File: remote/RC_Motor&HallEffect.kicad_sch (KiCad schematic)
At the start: 9 parts, among them P2 JST CONN, Q1 NMOS, SW4 Button, U4 TMAG5253

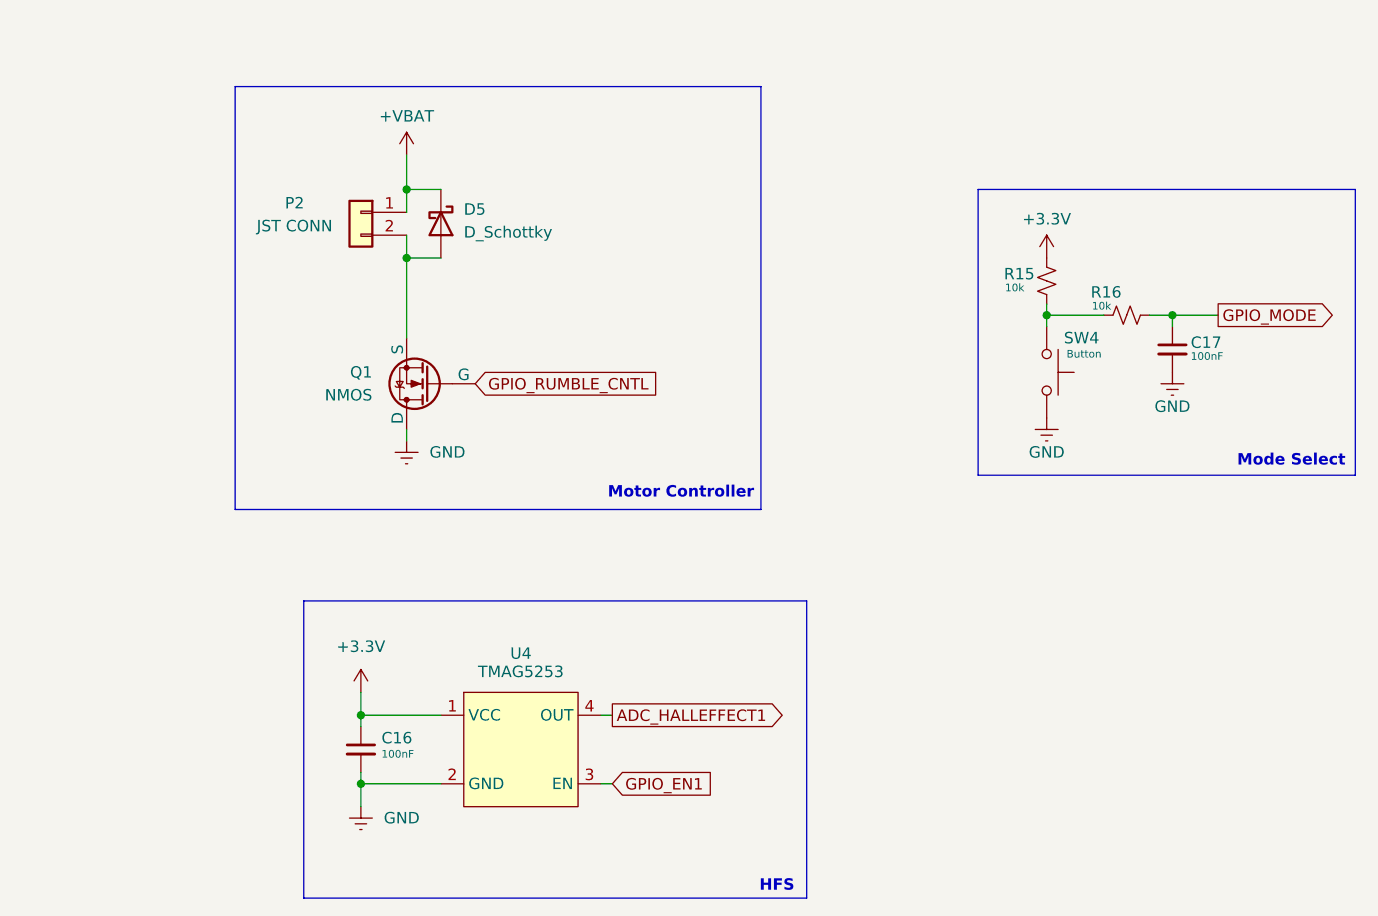
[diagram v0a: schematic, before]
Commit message: CRC V3
V 3.0.0
Initial version of CRC V3, fully redesigned remote
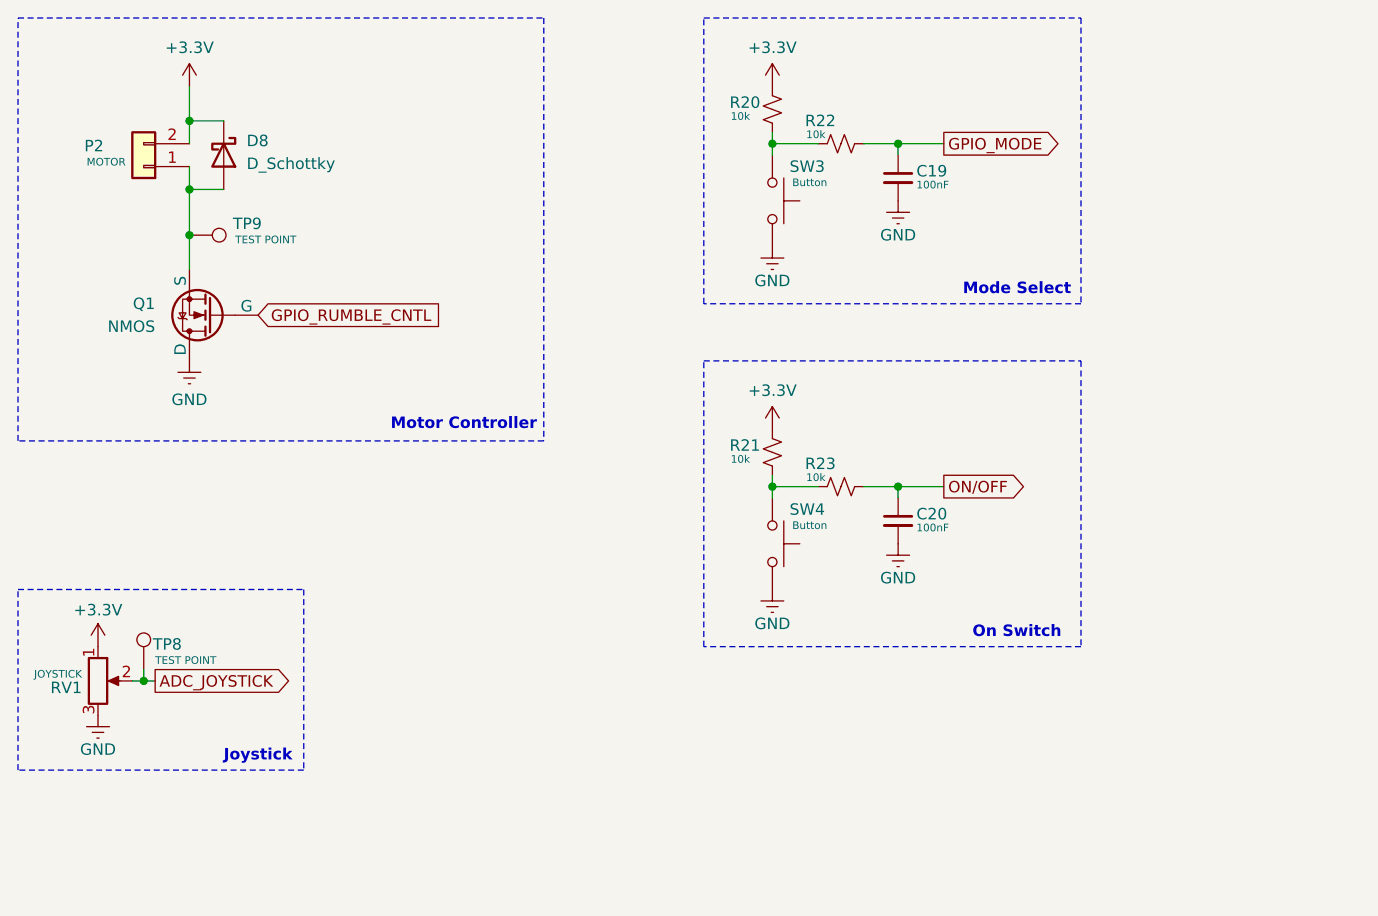
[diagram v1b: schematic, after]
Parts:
- removed C16: 100nF, Capacitor_SMD:C_0402_1005Metric, symbol Device:C_Small
- removed U4: TMAG5253, footprints:X2SON4_DMR_TEX, symbol New_Library_0:TMAG5253_Linear_Hall_Effect_Sensor
- added C20: 100nF, Capacitor_SMD:C_0402_1005Metric_Pad0.74x0.62mm_HandSolder, symbol Device:C_Small
- added R21, R23: 10k, Resistor_SMD:R_0402_1005Metric_Pad0.72x0.64mm_HandSolder, symbol Device:R_Small_US
- added RV1: JOYSTICK, footprints:Joystick Potentiometer Pads, symbol Device:R_Potentiometer
- added SW4: Button, footprints:Box Tactile Button Switch, symbol Switch:SW_Push
- added TP8, TP9: TEST POINT, TestPoint:TestPoint_Pad_2.0x2.0mm, symbol Connector:TestPoint
- C19: renamed from C17; footprint Capacitor_SMD:C_0402_1005Metric -> Capacitor_SMD:C_0402_1005Metric_Pad0.74x0.62mm_HandSolder
- P2: value JST CONN -> MOTOR; footprint footprints:CONN-SMD_2P-P2.00_XUNPU_WAFER-PH2.0-2PWB -> footprints:Motor Pads; LCSC# C3029440 -> (none); MPN C3029440 -> (none)
- R20: renamed from R15; footprint Resistor_SMD:R_0402_1005Metric -> Resistor_SMD:R_0402_1005Metric_Pad0.72x0.64mm_HandSolder
- R22: renamed from R16; footprint Resistor_SMD:R_0402_1005Metric -> Resistor_SMD:R_0402_1005Metric_Pad0.72x0.64mm_HandSolder
- SW3: renamed from SW4; footprint footprints:SW-SMD_L3.9-W3.0-P4.45 -> footprints:Box Tactile Button Switch; LCSC# C720477 -> (none); MPN C720477 -> (none)
- renumbered D5 to D8
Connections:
- net +3.3V: now also D8.1 (K), P2.2 (Pin_2), R21.1, RV1.1
- net GND: now also C20.2, RV1.3, SW4.2
- net at D8.2 (A), Q1.3 (S): now also P2.1 (Pin_1), TP9.1; no longer P2.2 (Pin_2)
- removed net +VBAT: D8.1 (K), P2.1 (Pin_1)
- new net: R21.2, R23.1, SW4.1
- new net ADC_JOYSTICK: RV1.2, TP8.1
- new net ON/OFF: C20.1, R23.2
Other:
- note added: "Joystick"
- note added: "On Switch"
- note removed: "HFS"
- moved on the sheet: C19, D8, P2, Q1, R20, R22, SW3
